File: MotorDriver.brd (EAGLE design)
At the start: 233.7 x 135.6 mm, 136 parts, among them IC3 STM32F071V8T6V8, J10 B4B-PH-K-S(LF)(SN), J11 B4B-PH-K-S(LF)(SN), J12 B4B-PH-K-S(LF)(SN), J13 B4B-PH-K-S(LF)(SN), J14 B4B-PH-K-S(LF)(SN), J15 B4B-PH-K-S(LF)(SN), J16 B4B-PH-K-S(LF)(SN), J18 B2P-VH(LF)(SN), J19 B2P-VH(LF)(SN), J20 B2P-VH(LF)(SN), J21 B2P-VH(LF)(SN), J22 B2P-VH(LF)(SN), J23 B2P-VH(LF)(SN), J24 B2P-VH(LF)(SN), J25 B2P-VH(LF)(SN), J26 XT30PWXT30PW, J9 B4B-PH-K-S(LF)(SN), M0 VNH7100ASTR, M1 VNH7100ASTR, M2 VNH7100ASTR, M3 VNH7100ASTR, M4 VNH7100ASTR, M5 VNH7100ASTR, M6 VNH7100ASTR, M7 VNH7100ASTR, Q2 20V/4.2A/52mΩ/1.4W, U1 ICE5LP1K-SG48ITR, U10 LD1085D2T33R, U11 LD1085D2T33R, U2 N25Q032A13ESC40F, U3 BD9D323QWZ-E2, U4 BD9D323QWZ-E2, U5 MMDT5401-7-F, U6 BD9D323QWZ-E2, U7 MIC5504-3.3YM5-TR, U8 MIC5365-1.2YC5-TR, U9 LD1085D2T33R, X1 MINI-USB-UX60-MB-5S8, Y1 ECS-TXO-2520-33-160-AN-TR

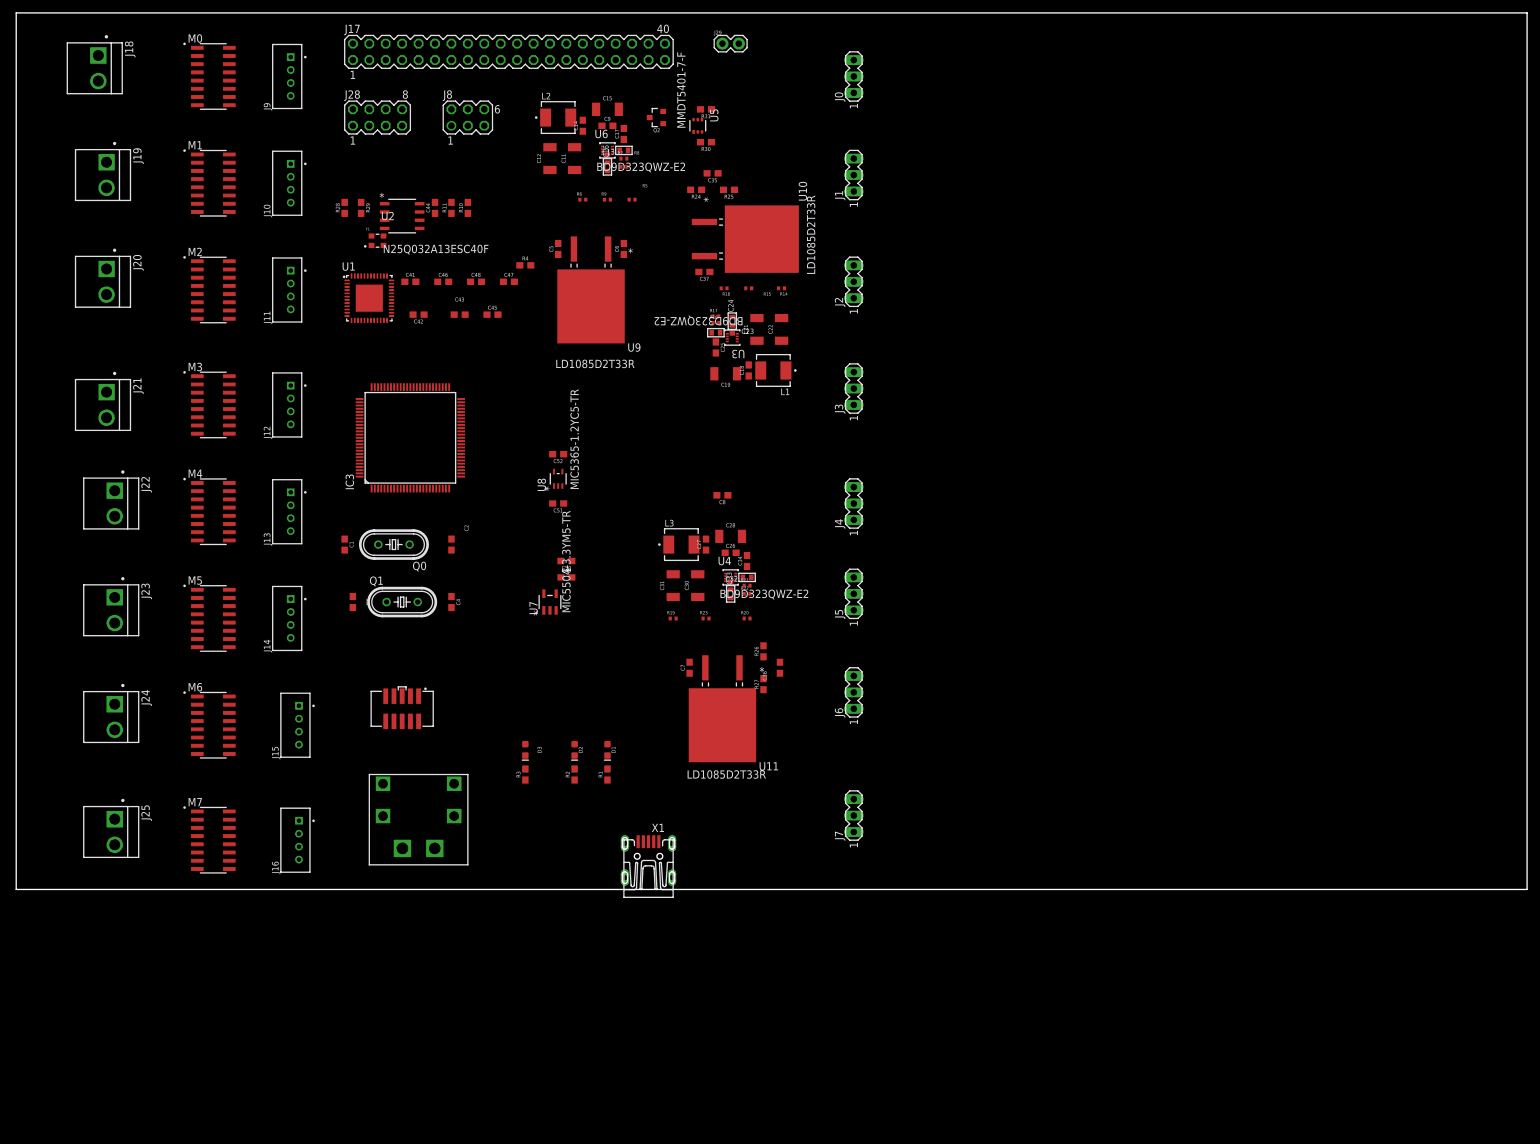
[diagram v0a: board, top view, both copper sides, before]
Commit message: Update
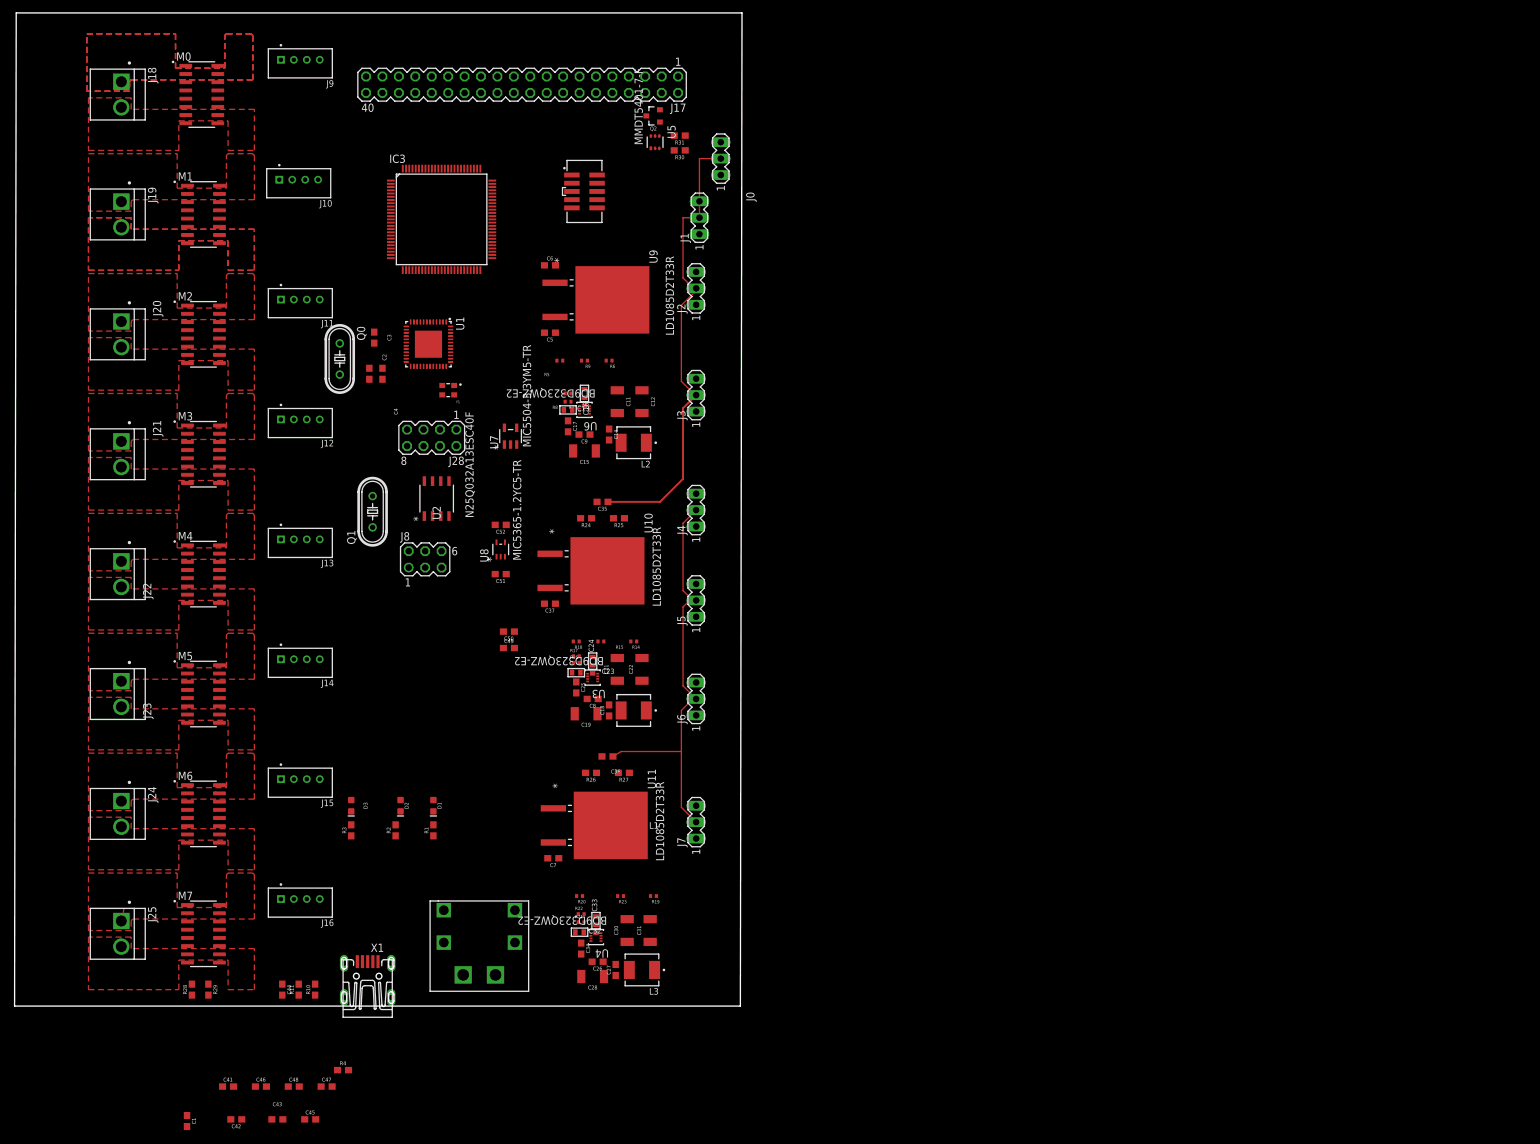
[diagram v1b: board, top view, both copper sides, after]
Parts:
- removed J29: (no value), SparkFun-Connectors:1X02
- moved C41 127.6 mm to (32.8, -30.5)
- moved C42 127.6 mm to (34.0, -35.6)
- moved C43 127.6 mm to (40.4, -35.6)
- moved C45 127.6 mm to (45.5, -35.6)
- moved C46 127.6 mm to (37.8, -30.5)
- moved C47 127.6 mm to (48.0, -30.5)
- moved C48 127.6 mm to (42.9, -30.5)
- moved R4 127.6 mm to (50.5, -27.9)
- moved C44 123.2 mm to (41.1, -15.5), turned to 270 degrees
- moved R10 123.2 mm to (46.2, -15.5)
- moved R11 123.2 mm to (43.7, -15.5)
- moved R28 123.2 mm to (27.2, -15.5)
- moved R29 123.2 mm to (29.7, -15.5)
- moved C1 92.4 mm to (26.4, -35.8)
- moved JTAG 84.8 mm to (87.9, 108.0), turned to 90 degrees
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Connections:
- removed net CRYTAL0_IN: IC3.8
- removed net EXTENAL_CLK: U1.35
- removed net N$19: JTAG.8
- removed net N$38: JTAG.6
- removed net N$5: C45.1, C47.1, R4.1, U1.29
- removed net N$6: J17.1
- new net FPGA_FLASH_CLK: J28.1, U1.15
- new net FPGA_FLASH_CS: J28.5, U1.16
- new net FPGA_FLASH_MISO: J28.3, U1.14
- new net FPGA_FLASH_MOSI: J28.7, U1.17
- net CRYSTAL0-IN: now also IC3.8
- net EXTERNAL_CLK: now also U1.35
- net FLASH_CLK: now also J28.2; no longer J28.1, U1.15
- net FLASH_CS: now also J28.6; no longer J28.2, U1.16
- net FLASH_HOLD: no longer J28.7
- net FLASH_MISO: now also J28.4; no longer J28.3, U1.14
- net FLASH_MOSI: now also J28.8; no longer J28.4, U1.17
- net FLASH_WP: no longer J28.8
- net FPGA_CDONE: now also IC3.34; no longer IC3.4
- net FPGA_CRESET_B: now also IC3.33; no longer IC3.3
- net FPGA_CS: now also IC3.35; no longer IC3.24
- net GND: now also C41.2, C42.2, C43.2, C45.2, C46.2, C47.2, C48.2; no longer J28.6, J29.2
- net M0_A: now also IC3.61; no longer IC3.67
- net M0_B: now also IC3.62; no longer IC3.68
- net M1_A: now also IC3.59; no longer IC3.69
- net M1_B: now also IC3.60; no longer IC3.70
- net M2_A: now also IC3.67; no longer IC3.71
- net M2_B: now also IC3.68; no longer IC3.2
- net M3_A: now also IC3.69; no longer IC3.1
- net M3_B: now also IC3.70; no longer IC3.77
- net M4_A: now also IC3.37; no longer IC3.23
- net M4_B: now also IC3.36; no longer IC3.25
- net M5_A: now also IC3.39; no longer IC3.26
- net M5_B: now also IC3.38; no longer IC3.29
- net M6_A: now also IC3.43; no longer IC3.38
- net M6_B: now also IC3.41; no longer IC3.39
- net M7_A: now also IC3.47; no longer IC3.41
- net M7_B: now also IC3.46; no longer IC3.43
- net RPI_5V: no longer J29.1
- net RPI_BUSY: now also IC3.48; no longer IC3.37
- net RPI_READY: now also IC3.58; no longer IC3.89
- net RPI_STATUS: now also IC3.55; no longer IC3.96
- net VCC_1_2V: now also C45.1, C47.1, R4.1, U1.29
- net VCC_3.3V: no longer C41.2, C42.2, C43.2, C45.2, C46.2, C47.2, C48.2, J17.17, J28.5
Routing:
- net SERVO_A_6V: track 0.00 -> 72.4 mm
- net SERVO_B_6V: track 0.00 -> 65.5 mm
- net GND: track 0.00 -> 6.66 mm
- net OUT7_A: track 0.00 -> 2.00 mm
- net OUT0_A: track 0.00 -> 0.63 mm
- added copper zone on layer 2, net GND
- added copper zone on layer 1, net OUT0_A
- added copper zone on layer 1, net OUT0_B
- added copper zone on layer 1, net OUT1_A
- added copper zone on layer 1, net OUT1_B
- added copper zone on layer 1, net OUT2_A
- added copper zone on layer 1, net OUT2_B
- added copper zone on layer 1, net OUT3_A
- added copper zone on layer 1, net OUT3_B
- added copper zone on layer 1, net OUT4_A
- added copper zone on layer 1, net OUT4_B
- added copper zone on layer 1, net OUT5_A
- added copper zone on layer 1, net OUT5_B
- added copper zone on layer 1, net OUT6_A
- added copper zone on layer 1, net OUT6_B
- added copper zone on layer 1, net OUT7_A
- added copper zone on layer 1, net OUT7_B
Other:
- board size 233.7 x 135.6 mm -> 112.5 x 153.6 mm

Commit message: update
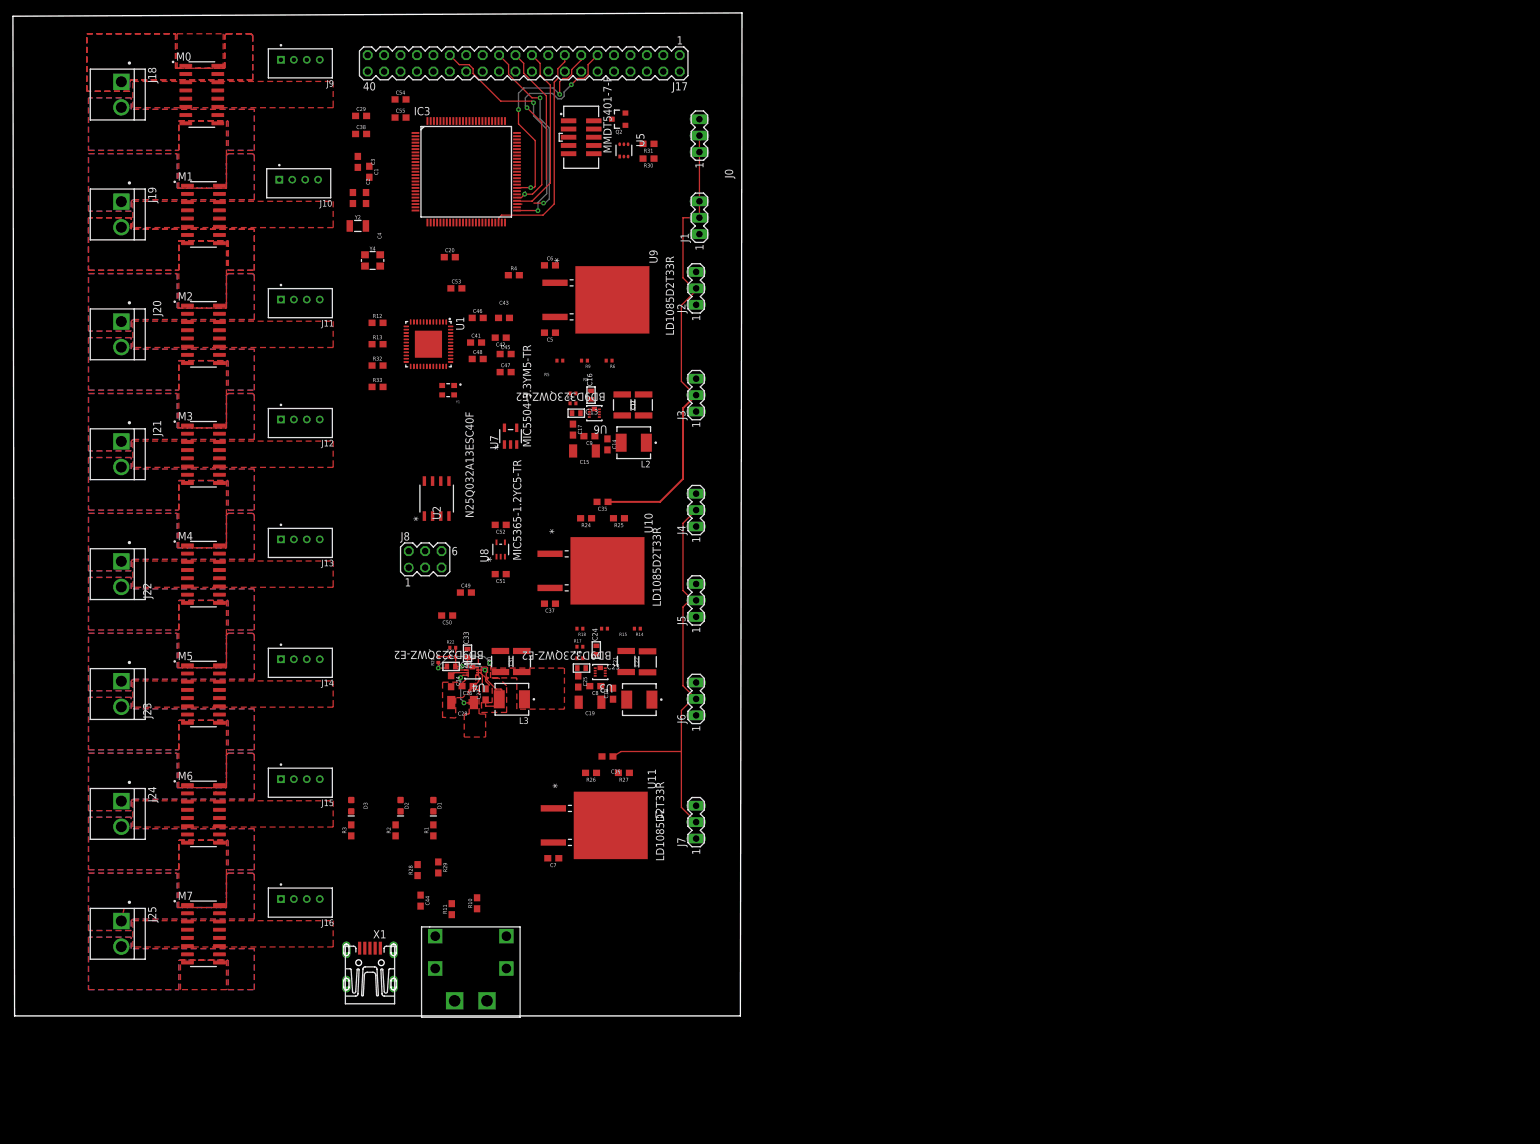
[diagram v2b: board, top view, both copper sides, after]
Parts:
- removed J28: (no value), con-lstb:MA04-2
- removed Q0, Q1: (no value), crystal:HC49/S
- added C20, C29, C38, C53, C54, C55: (no value), SparkFun-Capacitors:0603
- added R12, R13, R32, R33: 100, SparkFun-Resistors:0603
- added Y2: 32.768kHz, SparkFun-Clocks:CRYSTAL-SMD-3.2X1.5MM
- added Y4: CRYSTAL-GROUNDEDSMD-3.2X2.5, SparkFun-Clocks:CRYSTAL-SMD-3.2X2.5MM
- C11, C12, C21, C22, C30, C31: value 22UF-1210-16V-20% -> GRM32ER61E226KE15L; device SparkFun-Capacitors:1210 -> GRM32ER61E226KE15L:CAPC3225X270N
- moved C1 149.5 mm to (54.6, 111.0)
- moved C43 128.8 mm to (75.4, 88.4)
- moved C42 127.6 mm to (74.9, 85.3)
- moved R4 125.7 mm to (77.0, 95.0)
- moved C46 123.5 mm to (71.4, 88.4)
- moved C45 122.2 mm to (75.7, 82.8)
- moved C41 121.3 mm to (71.1, 84.6)
- moved C48 116.1 mm to (71.4, 82.0)
- moved C47 113.9 mm to (75.7, 80.0)
- moved C26 47.1 mm to (69.8, 31.4)
- moved C27 47.1 mm to (72.6, 30.2)
- moved C28 46.9 mm to (69.0, 28.9)
- moved R19 46.6 mm to (70.3, 36.0), flipped to the bottom
- moved L3 46.4 mm to (76.7, 29.4)
- moved C31 46.1 mm to (78.2, 35.3)
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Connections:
- new net 3.3V: C20.2, IC3.75
- new net CRYSTAL0_IN: C4.1, Y2.P$2
- new net N$5: C53.2, IC3.50
- net CRYSTAL0-IN: no longer C4.1, Q1.2
- net CRYSTAL0_OUT: now also Y2.P$1; no longer Q1.1
- net CRYSTAL1_IN: now also Y4.3; no longer Q0.2
- net CRYSTAL1_OUT: now also Y4.1; no longer Q0.1
- net FLASH_CLK: no longer J28.2
- net FLASH_CS: no longer J28.6
- net FLASH_MISO: no longer J28.4
- net FLASH_MOSI: no longer J28.8
- net FPGA_CLK: now also R13.2
- net FPGA_CS: now also R12.2
- net FPGA_FLASH_CLK: now also R13.1; no longer J28.1
- net FPGA_FLASH_CS: now also R12.1; no longer J28.5
- net FPGA_FLASH_MISO: now also R32.1; no longer J28.3
- net FPGA_FLASH_MOSI: now also R33.1; no longer J28.7
- net FPGA_MISO: now also R32.2
- net FPGA_MOSI: now also R33.2
- net GND: now also C20.1, C29.1, C38.1, C53.1, C54.1, C55.2, U4.9, Y4.2, Y4.4
- net VCC_3.3V: now also C29.2, C38.2, C54.2, C55.1; no longer IC3.50, IC3.75
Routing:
- net RPI_CS: track 0.00 -> 37.8 mm, vias 0 -> 2
- net RPI_STATUS: track 0.00 -> 35.9 mm, vias 0 -> 3
- net RPI_READY: track 0.00 -> 33.4 mm, vias 0 -> 3
- net RPI_BUSY: track 0.00 -> 33.4 mm
- net RPI_CLK: track 0.00 -> 28.9 mm, vias 0 -> 2
- net RPI_MOSI: track 0.00 -> 26.7 mm
- net RPI_MISO: track 0.00 -> 22.0 mm
- net N$32: track 0.00 -> 15.8 mm, vias 0 -> 1
- net N$30: track 0.00 -> 7.77 mm, vias 0 -> 1
- net N$35: track 0.00 -> 7.27 mm, vias 0 -> 1
- net VCC_12V: track 0.00 -> 6.94 mm, vias 0 -> 2
- net SERVO_B_6V: track 65.5 -> 69.7 mm, vias 0 -> 1
- net N$29: track 0.00 -> 3.28 mm
- net N$34: track 0.00 -> 2.72 mm
- net N$31: track 0.00 -> 1.80 mm
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- added copper zone on layer 1, net GND
- added copper zone on layer 1, net N$32
- added copper zone on layer 16, net OUT0_A
- added copper zone on layer 16, net OUT0_B
- added copper zone on layer 16, net OUT1_A
- added copper zone on layer 16, net OUT1_B
- added copper zone on layer 16, net OUT2_A
- added copper zone on layer 16, net OUT2_B
- added copper zone on layer 16, net OUT3_A
- added copper zone on layer 16, net OUT3_B
- added copper zone on layer 16, net OUT4_A
- added copper zone on layer 16, net OUT4_B
- added copper zone on layer 16, net OUT5_A
- added copper zone on layer 16, net OUT5_B
- added copper zone on layer 16, net OUT6_A
- added copper zone on layer 16, net OUT6_B
- added copper zone on layer 16, net OUT7_A
- added copper zone on layer 16, net OUT7_B
- added copper zone on layer 1, net SERVO_B_6V
- added copper zone on layer 1, net VCC_12V
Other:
- board size 112.5 x 153.6 mm -> 112.8 x 155.1 mm
